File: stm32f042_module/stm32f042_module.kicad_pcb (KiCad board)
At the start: 2 copper layers, 17 parts, among them P1 CONN_01X14, P2 CONN_01X04, P3 CONN_01X14, P4 CONN_01X03, SW1 RESET, U1 STM32F042F6P6, U2 APE8865U5-33-HF-3, X1 8.000Mhz

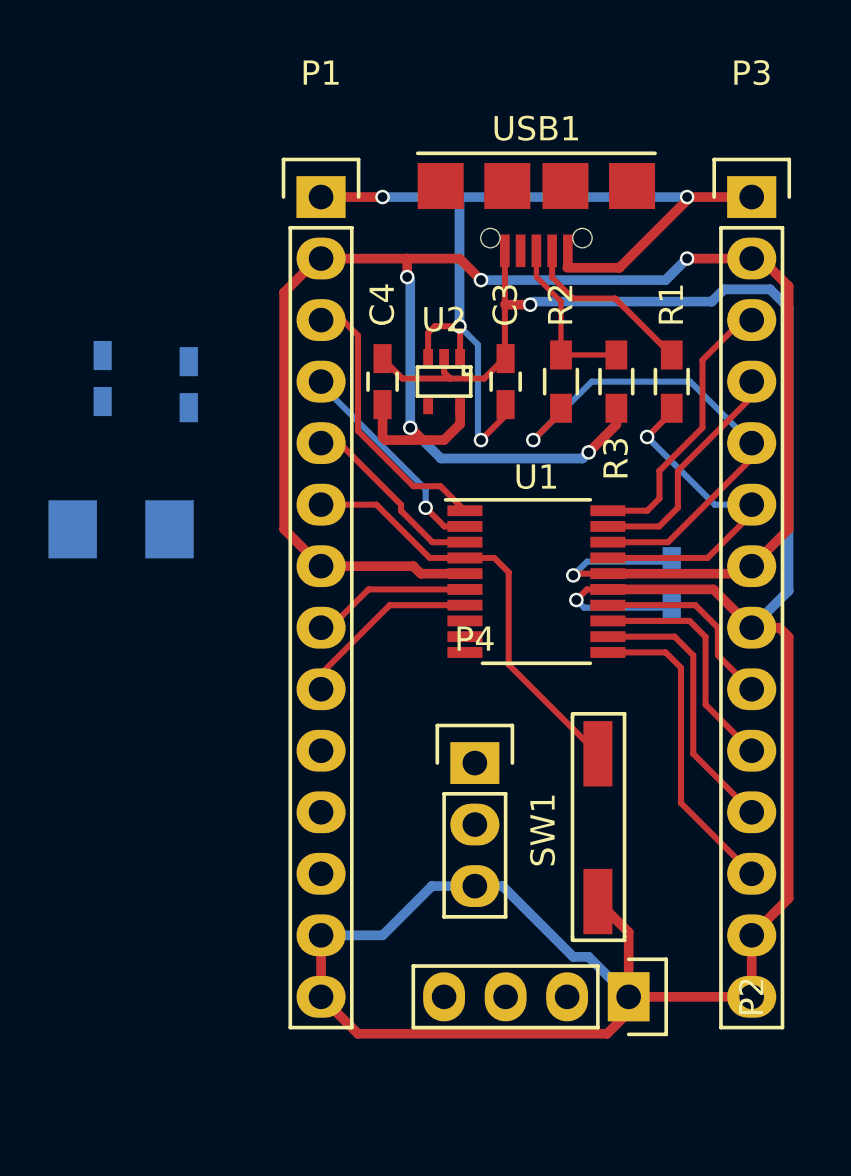
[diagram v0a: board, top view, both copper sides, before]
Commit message: final board
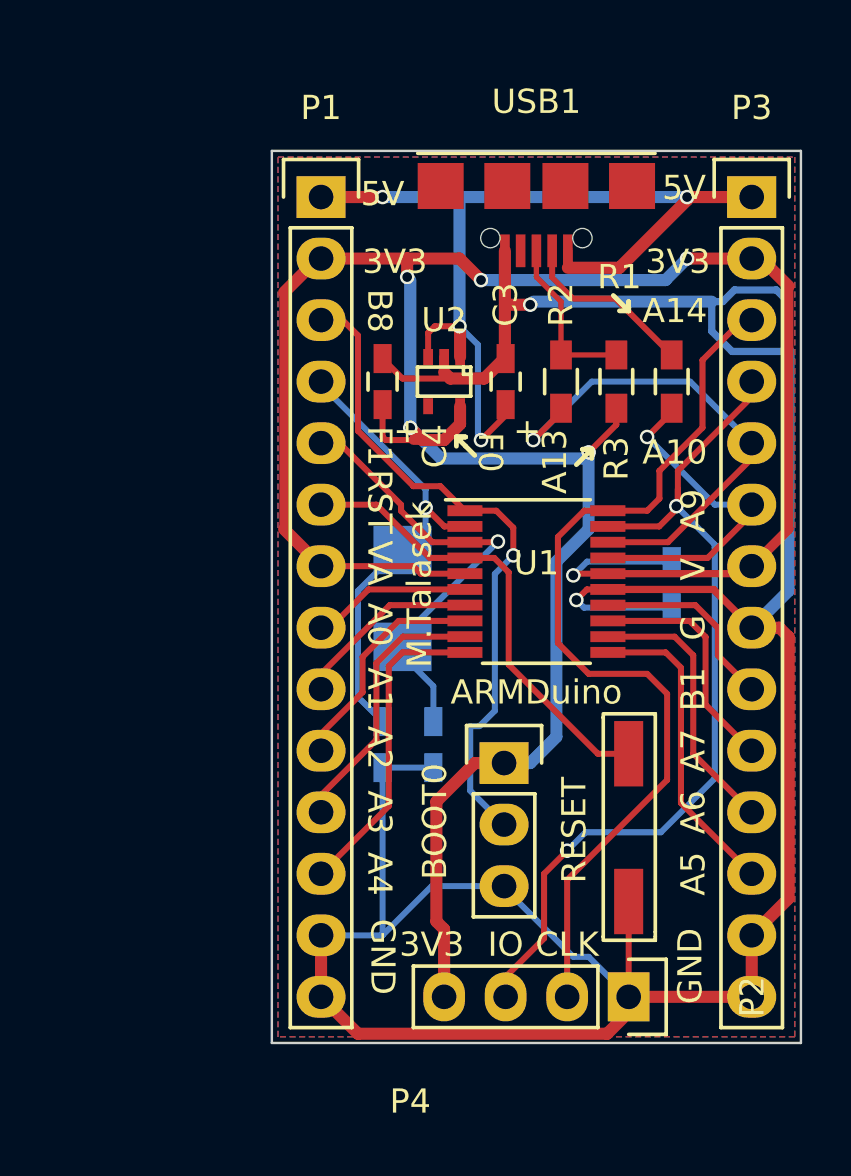
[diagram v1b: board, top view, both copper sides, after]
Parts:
- moved C2 19.0 mm to (134.6, 124.8)
- moved C1 18.0 mm to (136.7, 124.8), turned to 90 degrees
- moved X1 12.0 mm to (135.4, 118.8), turned to 270 degrees
- moved RESET 1.27 mm to (144.8, 128.3)
- moved P4 1.21 mm to (139.6, 125.6)
- renumbered SW1 to RESET
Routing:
- net Net-(P2-Pad3): track 9.68 -> 36.8 mm, vias 0 -> 2
- net +3V3: track 89.3 -> 115.8 mm
- net Net-(P2-Pad2): track 11.5 -> 38.0 mm
- net Net-(P1-Pad3): track 11.5 -> 27.6 mm, vias 0 -> 1
- net Net-(P1-Pad12): track 0.00 -> 13.1 mm
- net GND: track 108.6 -> 120.7 mm
- net Net-(P1-Pad11): track 0.00 -> 11.2 mm
- net Net-(C1-Pad2): track 7.78 -> 18.7 mm, vias 0 -> 1
- net Net-(C2-Pad2): track 9.19 -> 18.8 mm
- net Net-(P1-Pad10): track 0.00 -> 9.42 mm
- net Net-(P1-Pad6): track 17.9 -> 19.2 mm
- net +5V: track 40.0 -> 40.7 mm
- added copper zone on B.Cu, net GND
- added copper zone on F.Cu, net GND
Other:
- board outline added: 21.8 x 36.8 mm
- net class Power removed
- board text added: "+"
- board text added: "3V3"
- board text added: "5V"
- board text added: "A0"
- board text added: "A1"
- board text added: "A10"
- board text added: "A13"
- board text added: "A14"
- board text added: "A2"
- board text added: "A3"
- board text added: "A4"
- board text added: "A5"
- board text added: "A6"
- board text added: "A7"
- board text added: "A9"
- board text added: "ARMDuino"
- board text added: "B1"
- board text added: "B8"
- board text added: "BOOT0"
- board text added: "CLK"
- board text added: "F0"
- board text added: "F1"
- board text added: "G"
- board text added: "GND"
- board text added: "IO"
- board text added: "M.Talasek"
- board text added: "RST"
- board text added: "V"
- board text added: "VA"
